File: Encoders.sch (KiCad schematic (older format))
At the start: 2 parts, among them J7 Conn_01x04, J8 Conn_01x04

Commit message: Czyszczenie
Usunięto linie 5V oraz 2V8. Poprawiono symbol dla diody RGB
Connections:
- net labels added: +3V3
- net labels removed: +5V
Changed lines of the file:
@@
 ENC_R_B
 $Comp
-L power:+5V #PWR0170
-U 1 1 5E67CEDB
+L power:+3V3 #PWR0158
+U 1 1 5F70003D
 P 3600 2150
-F 0 "#PWR0170" H 3600 2000 50  0001 C CNN
-F 1 "+5V" H 3615 2323 50  0000 C CNN
+F 0 "#PWR0158" H 3600 2000 50  0001 C CNN
+F 1 "+3V3" H 3615 2323 50  0000 C CNN
 F 2 "" H 3600 2150 50  0001 C CNN
 F 3 "" H 3600 2150 50  0001 C CNN
@@
 $EndComp
 $Comp
-L power:+5V #PWR0172
-U 1 1 5E67D650
+L power:+3V3 #PWR0159
+U 1 1 5F700974
 P 3600 4300
-F 0 "#PWR0172" H 3600 4150 50  0001 C CNN
-F 1 "+5V" H 3615 4473 50  0000 C CNN
+F 0 "#PWR0159" H 3600 4150 50  0001 C CNN
+F 1 "+3V3" H 3615 4473 50  0000 C CNN
 F 2 "" H 3600 4300 50  0001 C CNN
 F 3 "" H 3600 4300 50  0001 C CNN

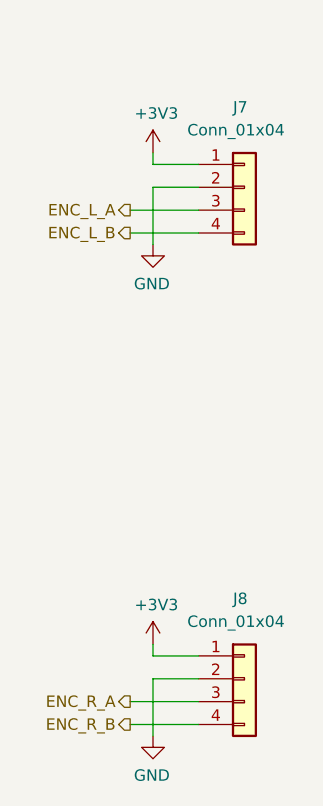
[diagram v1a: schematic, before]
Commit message: Holy $hi3t
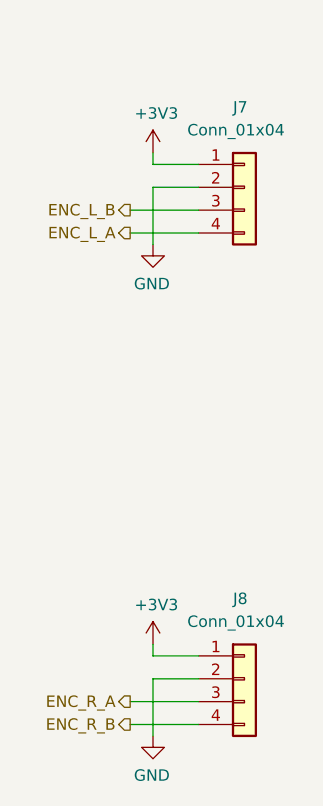
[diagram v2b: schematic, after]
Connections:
- net ENC_L_A: now also J7.4 (Pin_4); no longer J7.3 (Pin_3)
- net ENC_L_B: now also J7.3 (Pin_3); no longer J7.4 (Pin_4)
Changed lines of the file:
@@
 	-1   0    0    -1
 $EndComp
+Text HLabel 3500 2500 0    50   Output ~ 0
+ENC_L_A
 Text HLabel 3500 2400 0    50   Output ~ 0
-ENC_L_A
-Text HLabel 3500 2500 0    50   Output ~ 0
 ENC_L_B
 Text HLabel 3500 4550 0    50   Output ~ 0
